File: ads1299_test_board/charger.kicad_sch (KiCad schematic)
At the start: 10 parts, among them J1 Conn_01x02, Q1 AO3407A, U2 MCP73832-2-OT

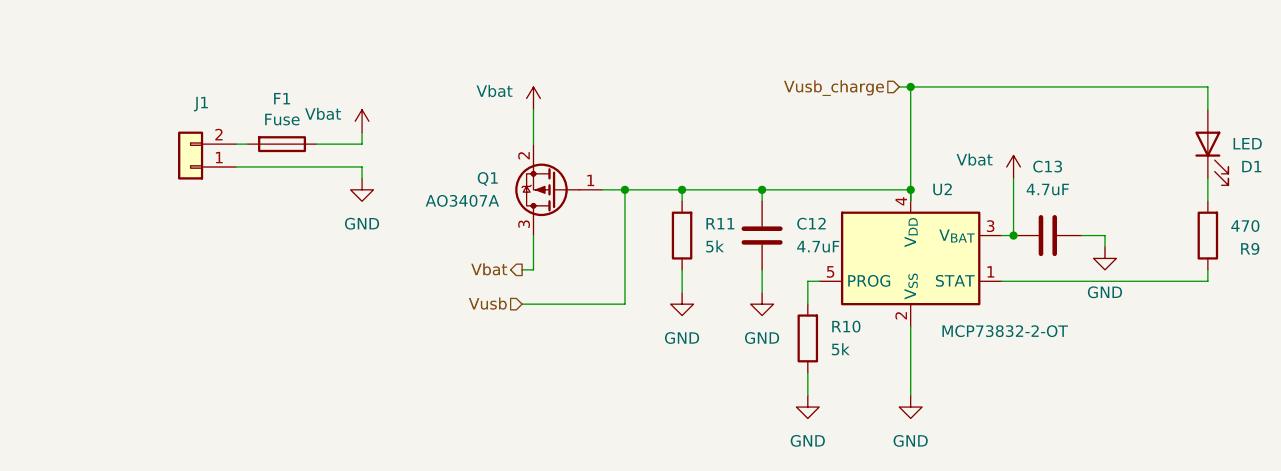
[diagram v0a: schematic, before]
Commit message: GPIO, SRB
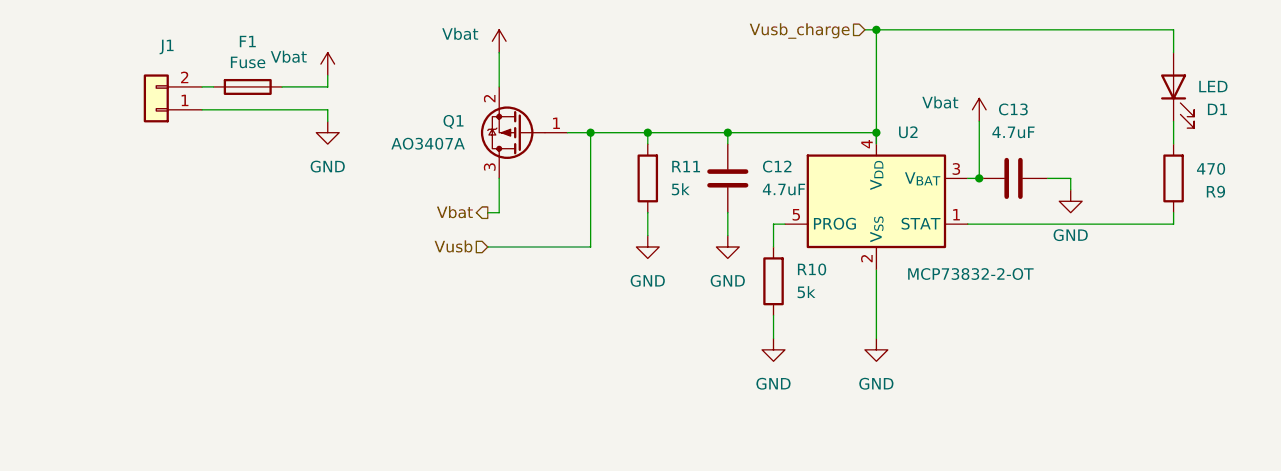
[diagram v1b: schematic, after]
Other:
- moved on the sheet: C12, C13, D1, F1, J1, Q1, R10, R11, R9, U2

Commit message: updates
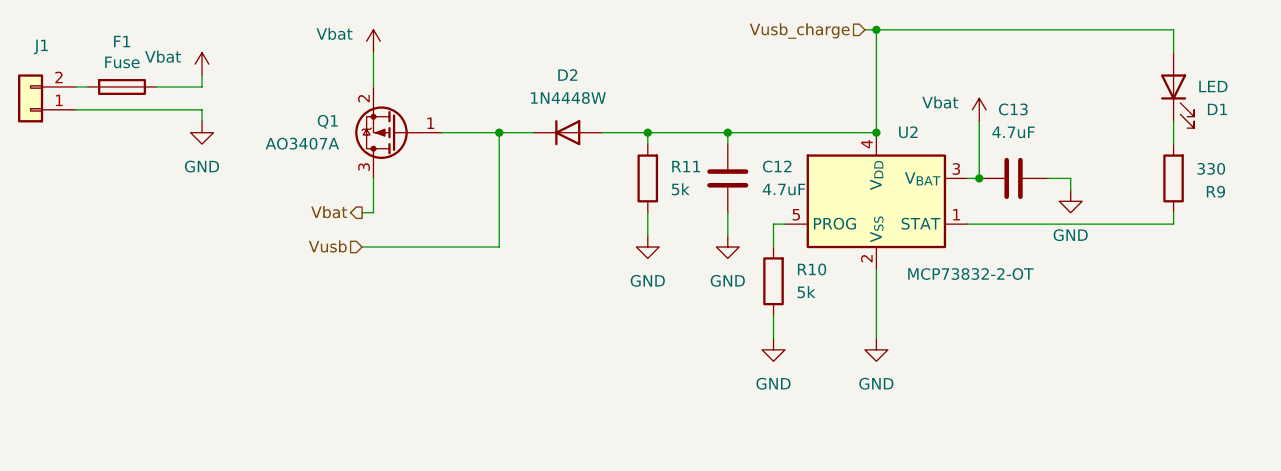
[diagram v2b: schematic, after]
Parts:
- added D2: 1N4448W, Diode_SMD:D_SOD-123, symbol Diode:1N4448W
- C12, C13, R10, R11: footprint (none) -> Capacitor_SMD:C_0402_1005Metric_Pad0.74x0.62mm_HandSolder
- D1: footprint (none) -> LED_SMD:LED_0603_1608Metric
- J1: footprint (none) -> Connector_JST:JST_EH_B2B-EH-A_1x02_P2.50mm_Vertical
- R9: value 470 -> 330; footprint (none) -> Capacitor_SMD:C_0402_1005Metric_Pad0.74x0.62mm_HandSolder
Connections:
- net Vusb: now also D2.1 (K); no longer C12.1, D1.2 (A), R11.2, U2.4 (V_{DD})
- new net Vusb_charge: C12.1, D1.2 (A), D2.2 (A), R11.2, U2.4 (V_{DD})
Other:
- moved on the sheet: F1, J1, Q1
